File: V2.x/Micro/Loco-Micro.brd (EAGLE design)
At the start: 16 x 15.9 mm, 30 parts, among them IC1 ATtiny25-20SSH, IC3 MCP1703CB

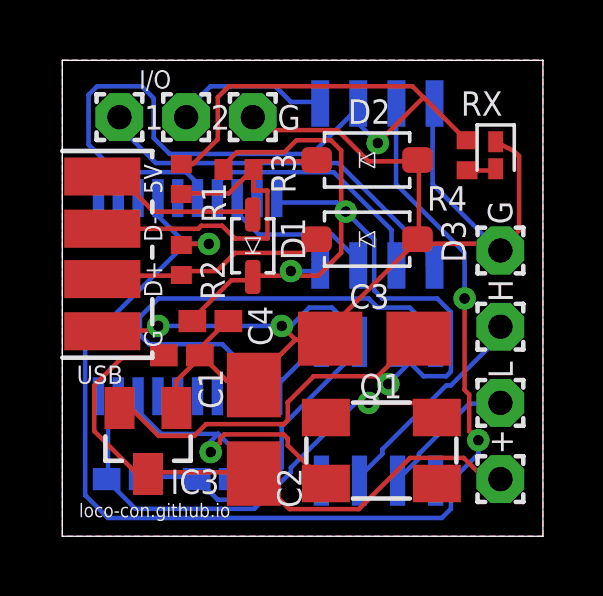
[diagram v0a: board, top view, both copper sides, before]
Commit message: updated micro module
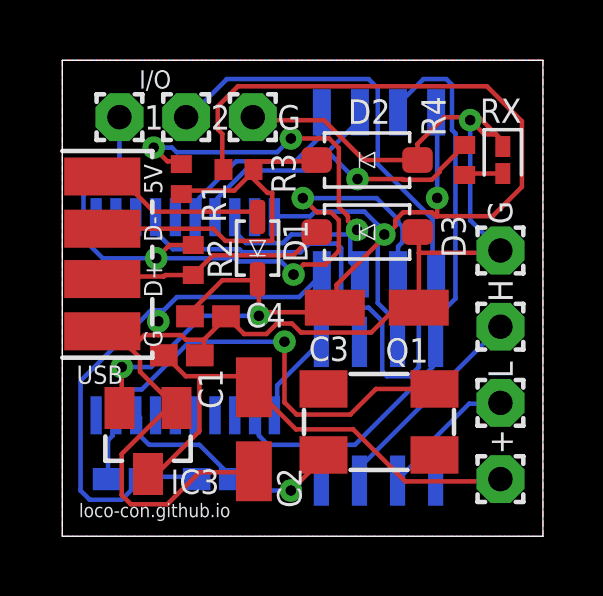
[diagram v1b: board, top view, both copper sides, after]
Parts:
- removed IC1: ATtiny25-20SSH, IC_Embedded:SOIC127P600X175-8N
- added IC2: ATtiny25-20SSH, ATtiny:SOIC127P600X175-8N
- C2, C3: device rcl:A/3216-18W -> rcl:CT3216
- moved C3 1.03 mm to (10.5, 7.62)
- moved Q1 0.96 mm to (10.6, 3.81)
- moved U$2 0.64 mm to (4.43, 7.33)
- moved R2 0.40 mm to (4.37, 9.21)
- moved RX 0.29 mm to (14.7, 12.5)
- moved D3 0.24 mm to (10.2, 10.1)
- moved D1 0.18 mm to (6.51, 9.60)
- moved R4 0.18 mm to (13.4, 12.5)
- moved C4 0.18 mm to (4.86, 7.33)
- renumbered PAD1 to +5V, PAD2 to D-, PAD3 to D+, PAD4 to GND
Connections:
- net CS: now also IC2.3, R1.2; no longer IC1.7
- net GND: now also IC2.4; no longer IC1.4
- net IO1: now also IC2.2, R2.2; no longer IC1.5
- net IO2: now also IC2.1; no longer IC1.1
- net SCK: now also IC2.7; no longer IC1.3, R2.2
- net SI: now also IC2.5; no longer IC1.2, R1.2, R4.2
- net SO: now also IC2.6, R4.2; no longer IC1.6
- net VCC: now also IC2.8; no longer IC1.8
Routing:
- net SI: track 34.0 -> 6.46 mm, vias 1 -> 0
- net SCK: track 41.0 -> 26.5 mm, vias 3 -> 0
- net CS: track 5.40 -> 17.1 mm, vias 0 -> 3
- net GND: track 56.4 -> 68.0 mm
- net IO1: track 13.0 -> 23.3 mm, vias 0 -> 3
- net IO2: track 5.23 -> 14.0 mm
- net N$7: track 16.6 -> 8.65 mm
- net VCC: track 41.7 -> 48.9 mm, vias 3 -> 4
- net SO: track 8.60 -> 12.4 mm, vias 0 -> 1
- net +12V: track 19.9 -> 17.2 mm
- net N$1: track 10.9 -> 8.19 mm
- net N$5: track 2.43 -> 3.10 mm
- net N$10: track 16.1 -> 16.7 mm
